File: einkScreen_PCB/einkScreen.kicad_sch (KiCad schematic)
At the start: 89 parts, among them J3 FH34SRJ-24S-0.5SH_50_, J4 UART, J5 5VPWR, Q1 A03400, Q2 A03401, Q3 S8050, Q4 A03401, Q5 A03401, SW1 SW_Push, SW2 SW_Push, SW3 SW_Push, SW4 SW_Push, U1 BQ51013BRHLR, U2 XC6220B331MR, U3 ESP32-C6-WROOM-1-N8

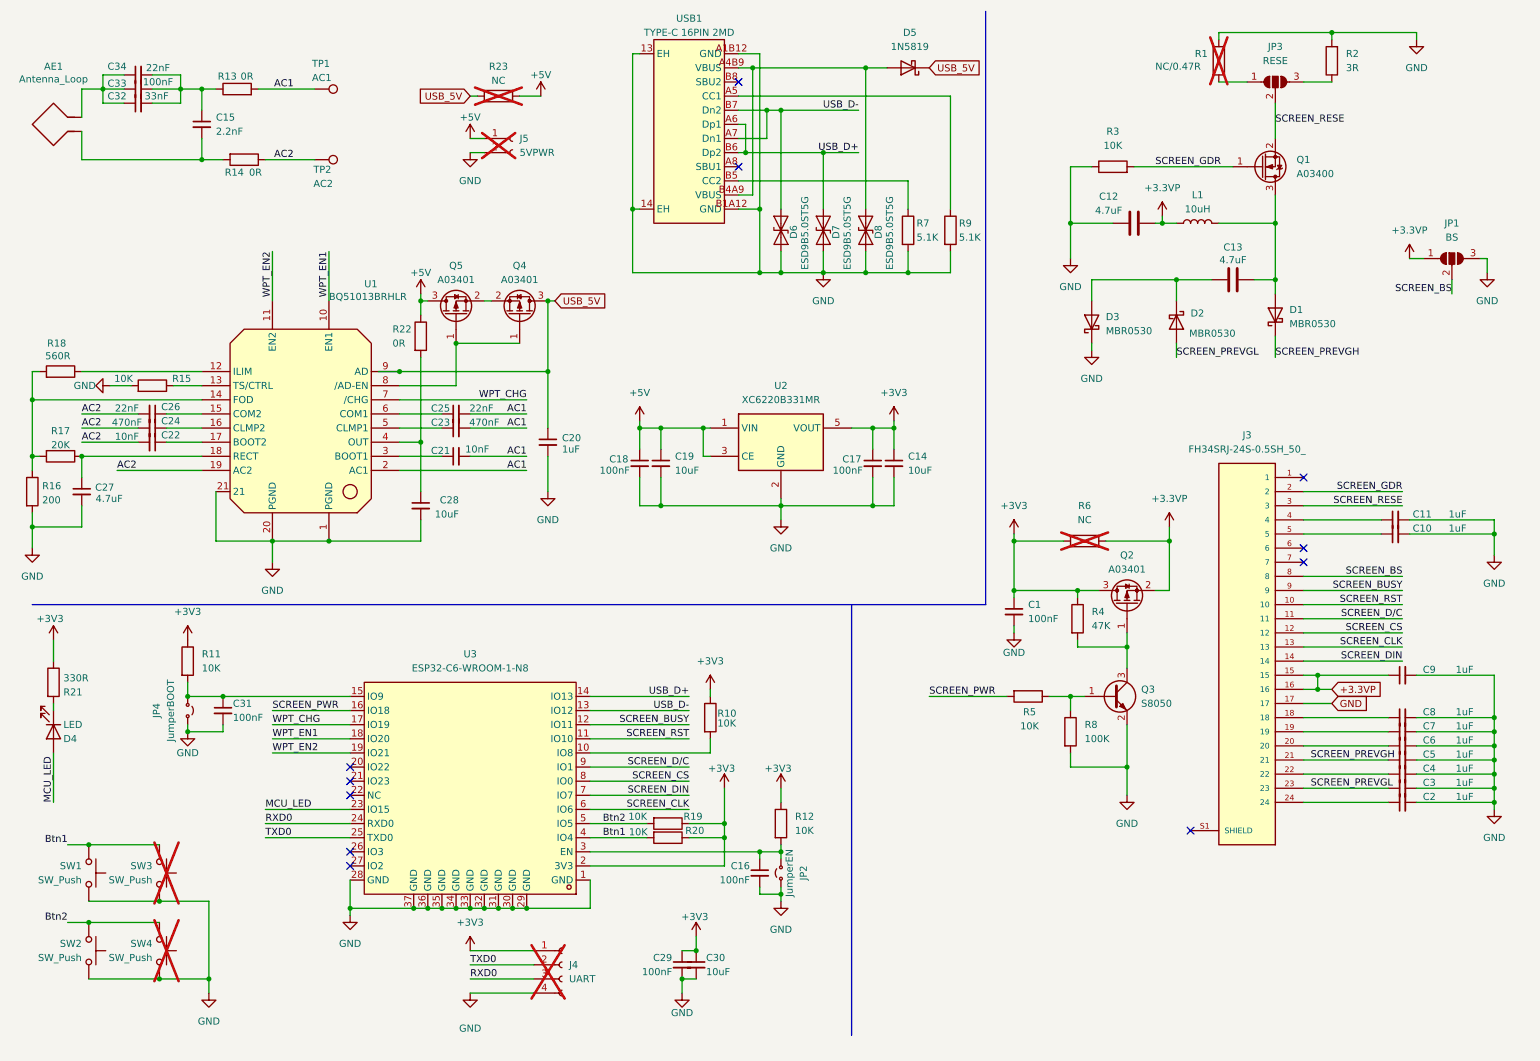
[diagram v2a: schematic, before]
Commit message: still working
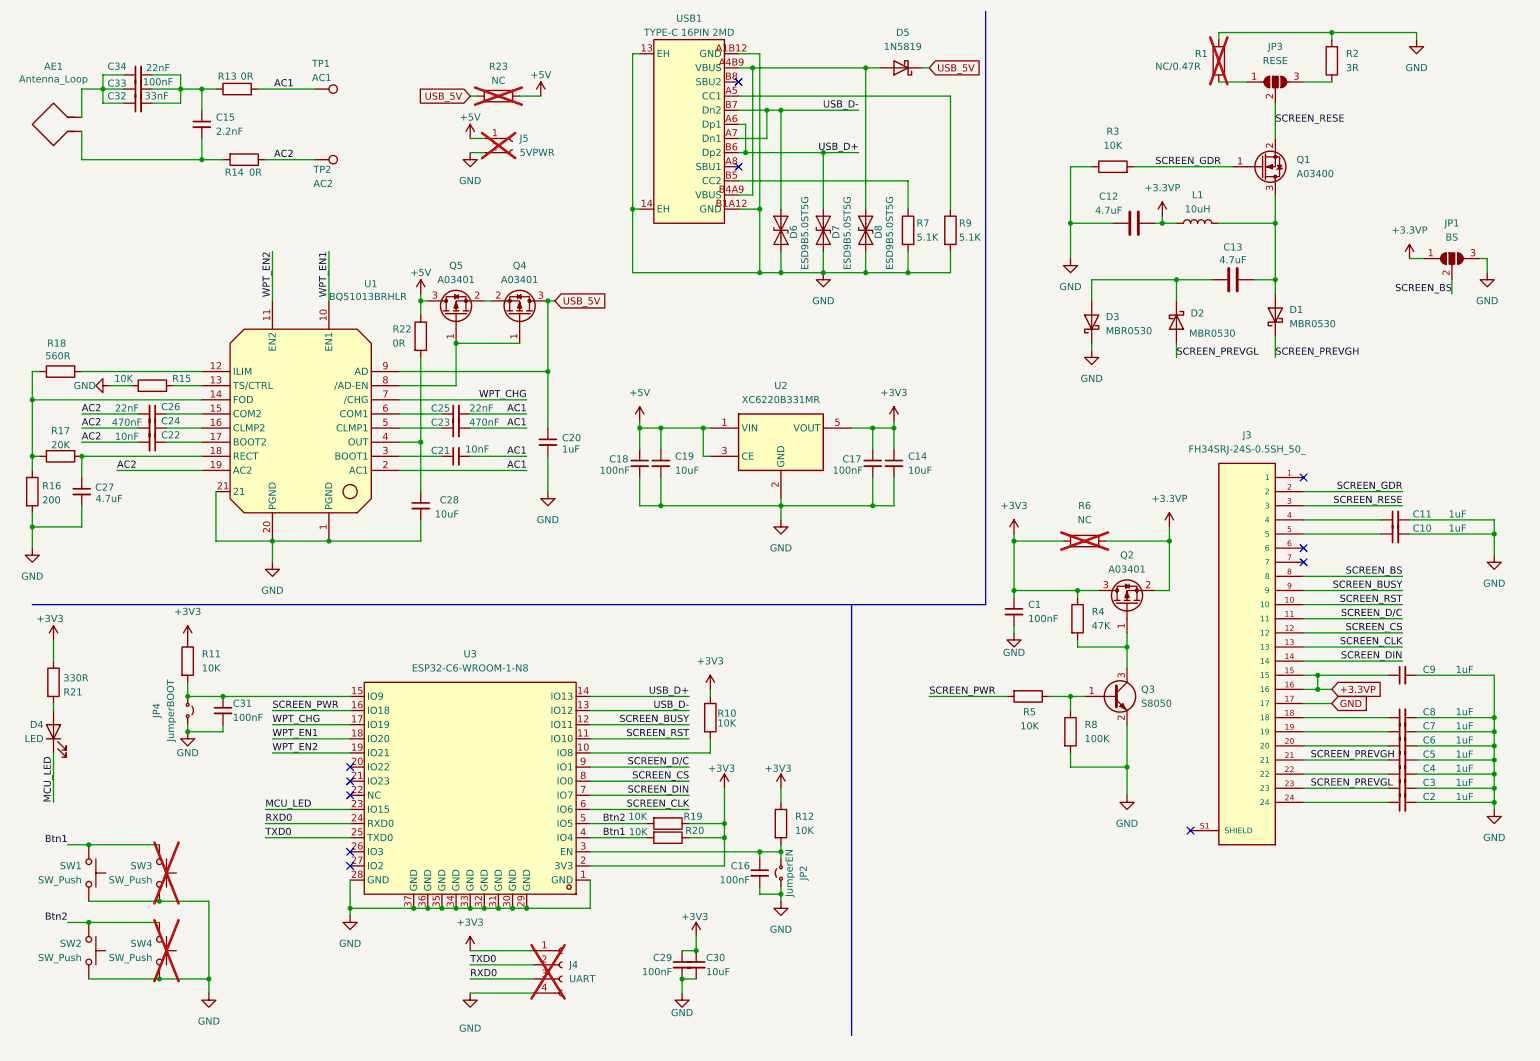
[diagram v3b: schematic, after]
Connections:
- net MCU_LED: now also D4.1 (K); no longer D4.2 (A)
- net at R21.2: now also D4.2 (A); no longer D4.1 (K)
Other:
- moved on the sheet: D4, D5
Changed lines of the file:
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@@
 	)
 	(junction
+		(at 165.1 22.86)
+		(diameter 0)
+		(color 0 0 0 0)
+	)
+	(junction
 		(at 27.94 26.67)
 		(diameter 0)
@@
 	)
 	(junction
-		(at 81.28 77.47)
-		(diameter 0)
-		(color 0 0 0 0)
-	)
-	(junction
 		(at 191.77 107.95)
 		(diameter 0)
@@
 	)
 	(junction
-		(at 165.1 22.86)
-		(diameter 0)
-		(color 0 0 0 0)
-	)
-	(junction
 		(at 43.18 142.24)
 		(diameter 0)
@@
 	(wire
 		(pts
+			(xy 19.05 137.16) (xy 19.05 138.43)
+		)
+		(stroke
+			(width 0)
+			(type default)
+		)
+	)
+	(wire
+		(pts
 			(xy 201.93 57.15) (xy 201.93 50.8)
 		)
@@
 	(wire
 		(pts
-			(xy 165.1 22.86) (xy 168.91 22.86)
+			(xy 165.1 22.86) (xy 167.64 22.86)
 		)
 		(stroke
@@
 	(wire
 		(pts
-			(xy 19.05 137.16) (xy 19.05 138.43)
-		)
-		(stroke
-			(width 0)
-			(type default)
-		)
-	)
-	(wire
-		(pts
 			(xy 243.84 147.32) (xy 259.08 147.32)
 		)
@@
 	(wire
 		(pts
+			(xy 175.26 22.86) (xy 176.53 22.86)
+		)
+		(stroke
+			(width 0)
+			(type default)
+		)
+	)
+	(wire
+		(pts
 			(xy 25.4 172.72) (xy 38.1 172.72)
 		)
@@
 	(wire
 		(pts
-			(xy 77.47 77.47) (xy 81.28 77.47)
+			(xy 142.24 33.02) (xy 143.51 33.02)
 		)
 		(stroke
@@
 	(wire
 		(pts
-			(xy 142.24 33.02) (xy 143.51 33.02)
+			(xy 115.57 158.75) (xy 125.73 158.75)
 		)
 		(stroke
@@
 	(wire
 		(pts
-			(xy 115.57 158.75) (xy 125.73 158.75)
+			(xy 128.27 87.63) (xy 128.27 91.44)
 		)
 		(stroke
@@
 	(wire
 		(pts
-			(xy 128.27 87.63) (xy 128.27 91.44)
+			(xy 203.2 127) (xy 203.2 125.73)
 		)
 		(stroke
@@
 	(wire
 		(pts
-			(xy 203.2 127) (xy 203.2 125.73)
+			(xy 25.4 162.56) (xy 38.1 162.56)
 		)
 		(stroke
@@
 	(wire
 		(pts
-			(xy 25.4 162.56) (xy 38.1 162.56)
+			(xy 49.53 135.89) (xy 72.39 135.89)
 		)
 		(stroke
@@
 	(wire
 		(pts
-			(xy 49.53 135.89) (xy 72.39 135.89)
+			(xy 203.2 116.84) (xy 207.01 116.84)
 		)
 		(stroke
@@
 	(wire
 		(pts
-			(xy 203.2 116.84) (xy 207.01 116.84)
+			(xy 19.05 146.05) (xy 19.05 154.94)
 		)
 		(stroke
@@
 	(wire
 		(pts
-			(xy 19.05 146.05) (xy 19.05 154.94)
-		)
-		(stroke
-			(width 0)
-			(type default)
-		)
-	)
-	(wire
-		(pts
 			(xy 246.38 132.08) (xy 259.08 132.08)
 		)
@@
 		)
 	)
+	(netclass_flag ""
+		(length 2.54)
+		(shape round)
+		(at 96.52 64.77 0)
+		(effects
+			(font
+				(size 1.27 1.27)
+			)
+			(justify left bottom)
+		)
+		(property "Net Class" "Power"
+			(at 94.234 65.786 0)
+			(show_name no)
+			(do_not_autoplace no)
+			(effects
+				(font
+					(size 1.27 1.27)
+				)
+				(justify left)
+			)
+		)
+		(property "Component Class" ""
+			(at -104.14 49.53 0)
+			(show_name no)
+			(do_not_autoplace no)
+			(effects
+				(font
+					(size 1.27 1.27)
+					(italic yes)
+				)
+			)
+		)
+	)
 	(symbol
 		(lib_id "power:+3V3")
@@
 	(symbol
 		(lib_id "Device:D_Schottky")
-		(at 172.72 22.86 180)
+		(at 171.45 22.86 180)
 		(unit 1)
 		(body_style 1)
@@
 		(fields_autoplaced yes)
 		(property "Reference" "D5"
-			(at 173.0375 16.51 0)
+			(at 171.7675 16.51 0)
 			(show_name no)
 			(do_not_autoplace no)
@@
 		)
 		(property "Value" "1N5819"
-			(at 173.0375 19.05 0)
+			(at 171.7675 19.05 0)
 			(show_name no)
 			(do_not_autoplace no)
@@
 		)
 		(property "Footprint" "Diode_SMD:D_SOD-123"
-			(at 172.72 22.86 0)
+			(at 171.45 22.86 0)
 			(hide yes)
 			(show_name no)
@@
 		)
 		(property "Datasheet" ""
-			(at 172.72 22.86 0)
+			(at 171.45 22.86 0)
 			(hide yes)
 			(show_name no)
@@
 		)
 		(property "Description" "Schottky diode"
-			(at 172.72 22.86 0)
+			(at 171.45 22.86 0)
 			(hide yes)
 			(show_name no)
@@
 		)
 		(property "PARTREV" ""
-			(at 172.72 22.86 0)
+			(at 171.45 22.86 0)
 			(hide yes)
 			(show_name no)
@@
 		)
 		(property "STANDARD" ""
-			(at 172.72 22.86 0)
+			(at 171.45 22.86 0)
 			(hide yes)
 			(show_name no)
@@
 		)
 		(property "Sim.Type" ""
-			(at 172.72 22.86 0)
+			(at 171.45 22.86 0)
 			(hide yes)
 			(show_name no)
@@
 		)
 		(property "LCSC" "C82544"
-			(at 172.72 22.86 0)
+			(at 171.45 22.86 0)
 			(hide yes)
 			(show_name no)
@@
 	(symbol
 		(lib_id "Device:LED")
-		(at 19.05 142.24 270)
+		(at 19.05 142.24 90)
 		(unit 1)
 		(body_style 1)
@@
 		(dnp no)
 		(property "Reference" "D4"
-			(at 20.828 143.51 90)
+			(at 17.272 140.97 90)
 			(show_name no)
 			(do_not_autoplace no)
@@
 		)
 		(property "Value" "LED"
-			(at 20.828 140.97 90)
+			(at 17.272 143.51 90)
 			(show_name no)
 			(do_not_autoplace no)

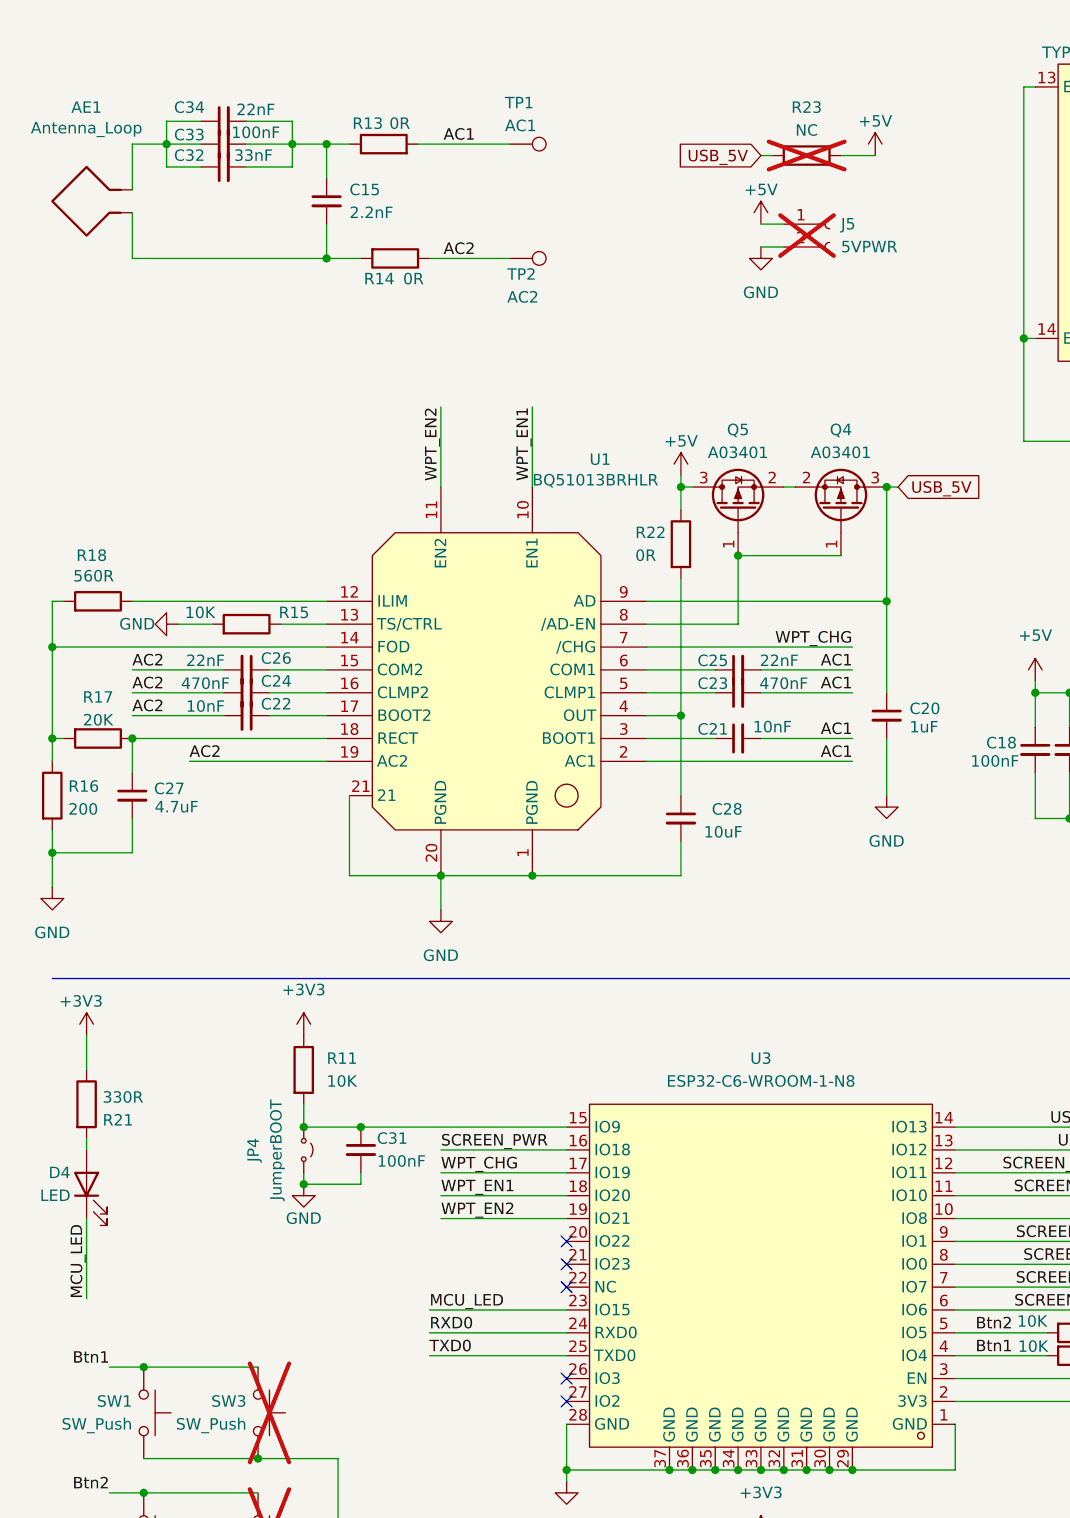
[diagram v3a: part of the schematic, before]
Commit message: fixed card issues
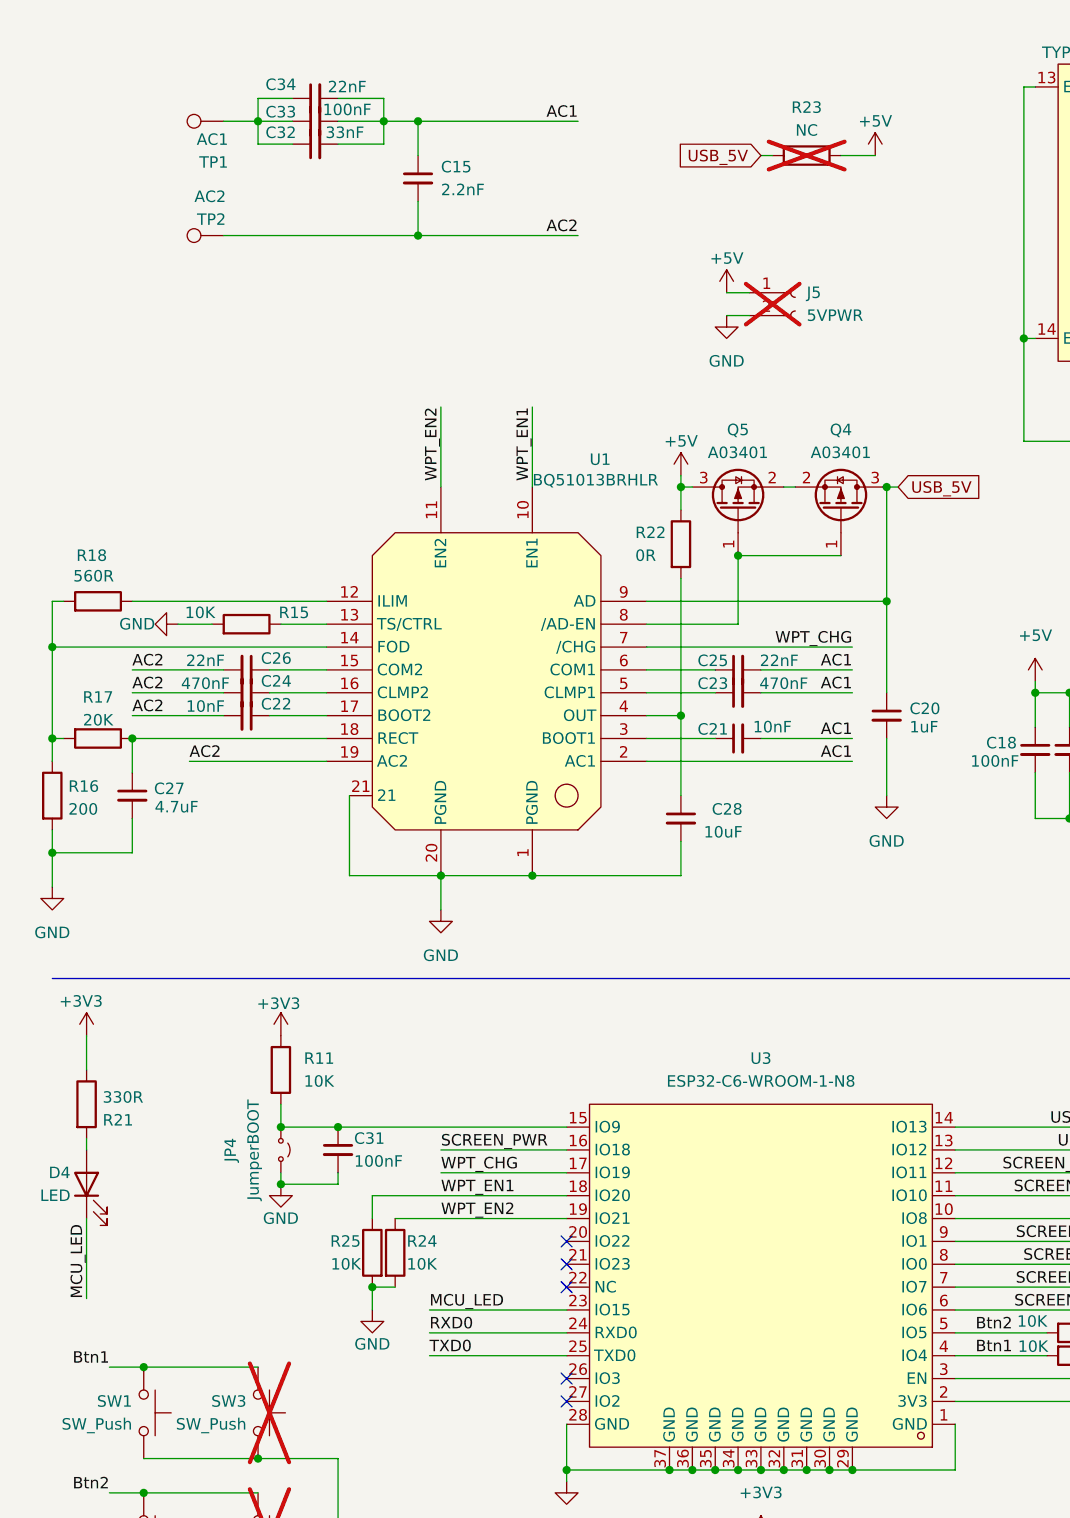
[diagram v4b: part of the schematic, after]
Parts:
- removed AE1: Antenna_Loop, PCB Coils:WPT_COIL, symbol Device:Antenna_Loop
- removed R13, R14: 0R, Resistor_SMD:R_0805_2012Metric, symbol Device:R
- added R24, R25: 10K, Resistor_SMD:R_0805_2012Metric, symbol Device:R
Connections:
- net AC1: now also C15.1, C32.2, C33.2, C34.2; no longer TP1.1
- net AC2: now also C15.2
- net GND: now also R24.2, R25.2
- net WPT_EN1: now also R25.1
- net WPT_EN2: now also R24.1
- net at C32.1, C33.1, C34.1: now also TP1.1
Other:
- moved on the sheet: C15, C31, C32, C33, C34, J5, JP4, R11, TP1, TP2
